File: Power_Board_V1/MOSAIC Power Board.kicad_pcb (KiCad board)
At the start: 2 copper layers, 89 x 89 mm, 41 parts, among them J1 CONN E, J10 CONN 2MM JST, J11 CONN 2MM JST, J12 CONN 2MM JST, J13 CONN 2MM JST, J14 CONN 2MM JST, J15 CONN 2MM JST, J16 CONN_JST_BATT, J2 CONN_QWIIC, J3 CONN_JST_BATT, J4 CONN 2MM JST, J5 CONN 2MM JST, J6 CONN 2MM JST, J7 CONN 2MM JST, J8 CONN 2MM JST, J9 CONN 2MM JST, U1 INA219, U2 INA219, U3 INA219, U4 INA219, U5 INA219, U6 INA219, U7 INA219

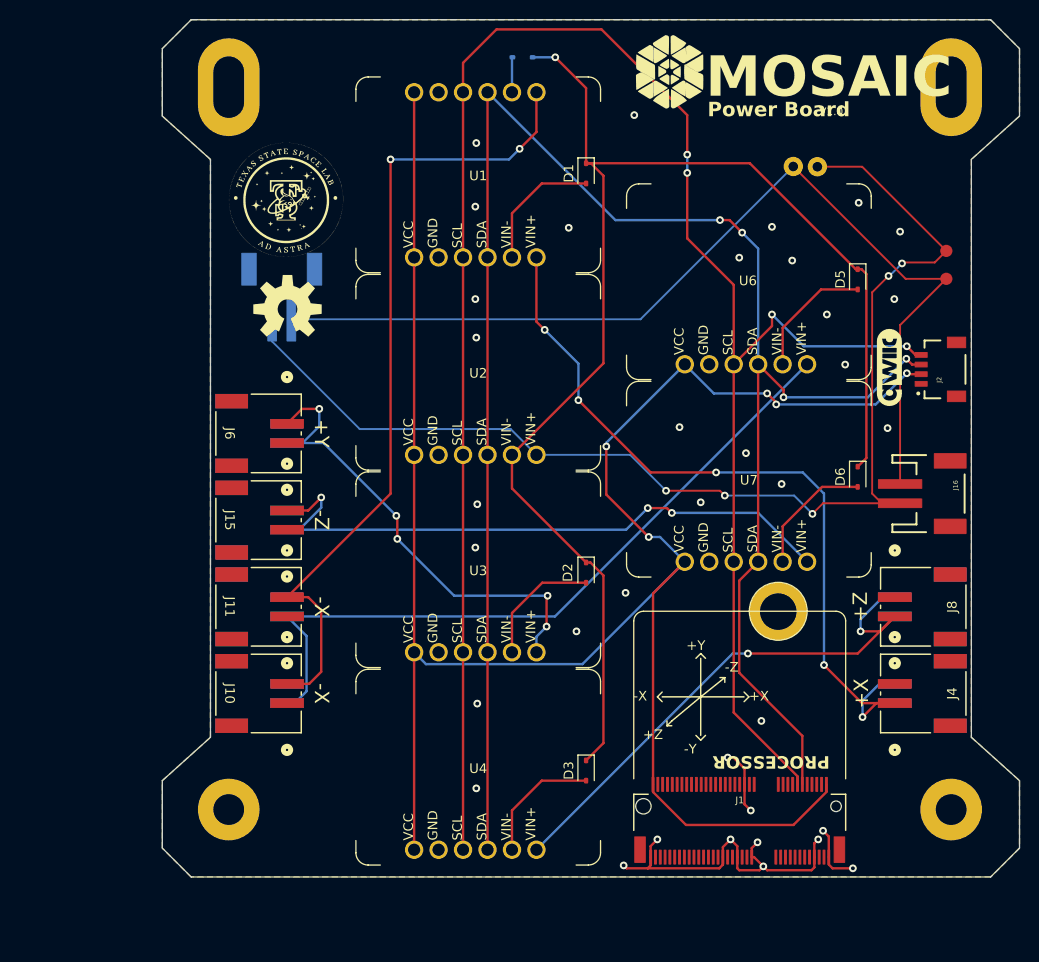
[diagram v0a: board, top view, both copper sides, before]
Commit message: Made JLCPCB production files
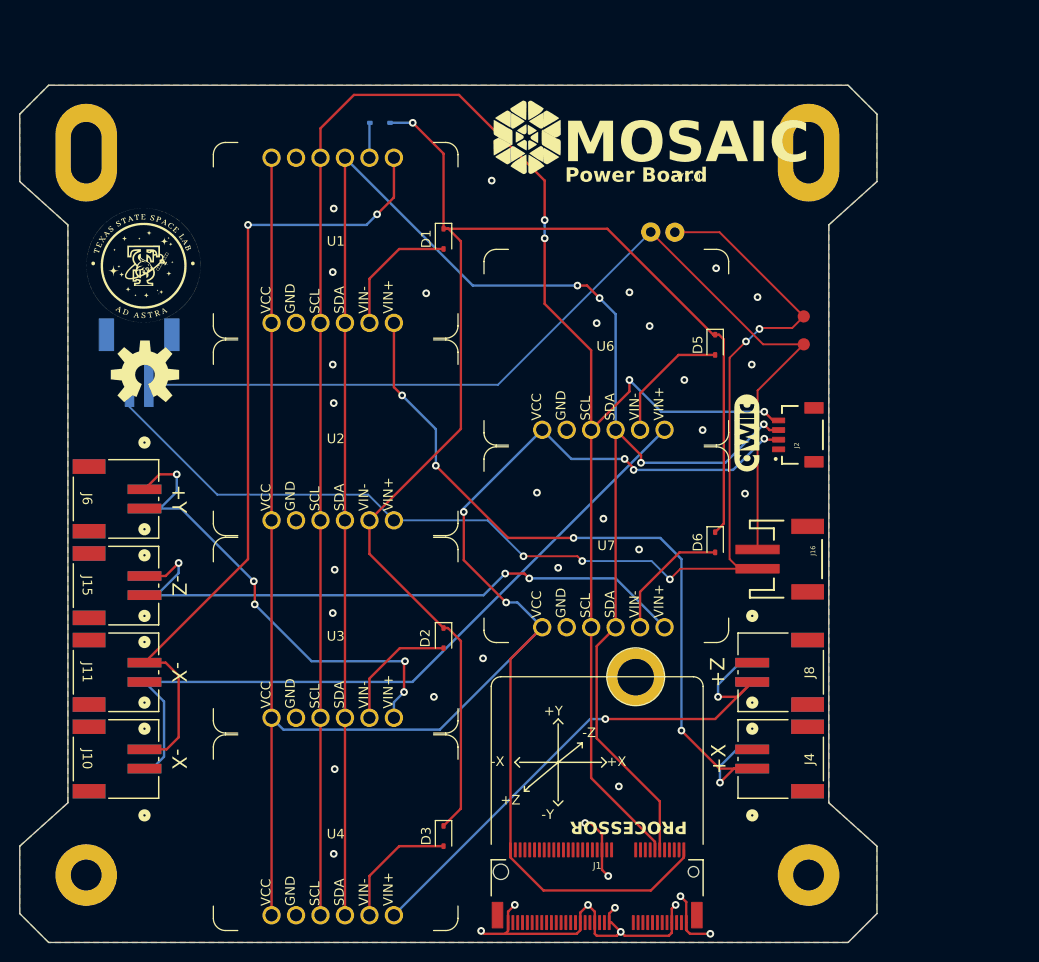
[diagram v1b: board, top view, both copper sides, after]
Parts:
- LOGO1: value QWIIC_LOGO_8MM -> ~
- LOGO2: value OSHW-LOGOL -> ~
- moved D3 16.3 mm to (136.7, 134.6)
- moved BT1 16.3 mm to (136.0, 108.5)
- moved D1 16.3 mm to (136.7, 72.5)
- moved D2 16.3 mm to (136.7, 114.0)
- moved D4 16.3 mm to (130.1, 60.5)
- moved H10 16.3 mm to (174.6, 63.6)
- moved H9 16.3 mm to (99.6, 63.6)
- moved J10 16.3 mm to (102.7, 126.5)
- moved J11 16.3 mm to (102.7, 117.5)
- moved J12 16.3 mm to (102.7, 126.5)
- moved J13 16.3 mm to (102.7, 117.5)
- moved J14 16.3 mm to (102.7, 108.5)
- moved J15 16.3 mm to (102.7, 108.5)
- moved J16 16.3 mm to (173.0, 105.8)
- moved J3 16.3 mm to (105.1, 84.0)
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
